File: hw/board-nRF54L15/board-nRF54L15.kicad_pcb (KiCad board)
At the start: 2 copper layers, 30 x 42 mm, 17 parts, among them J1 JST-PH 2.0 / BATTERY, SW1 B3U-1000P, U1 XIAO nRF54L15, U2 BMA400

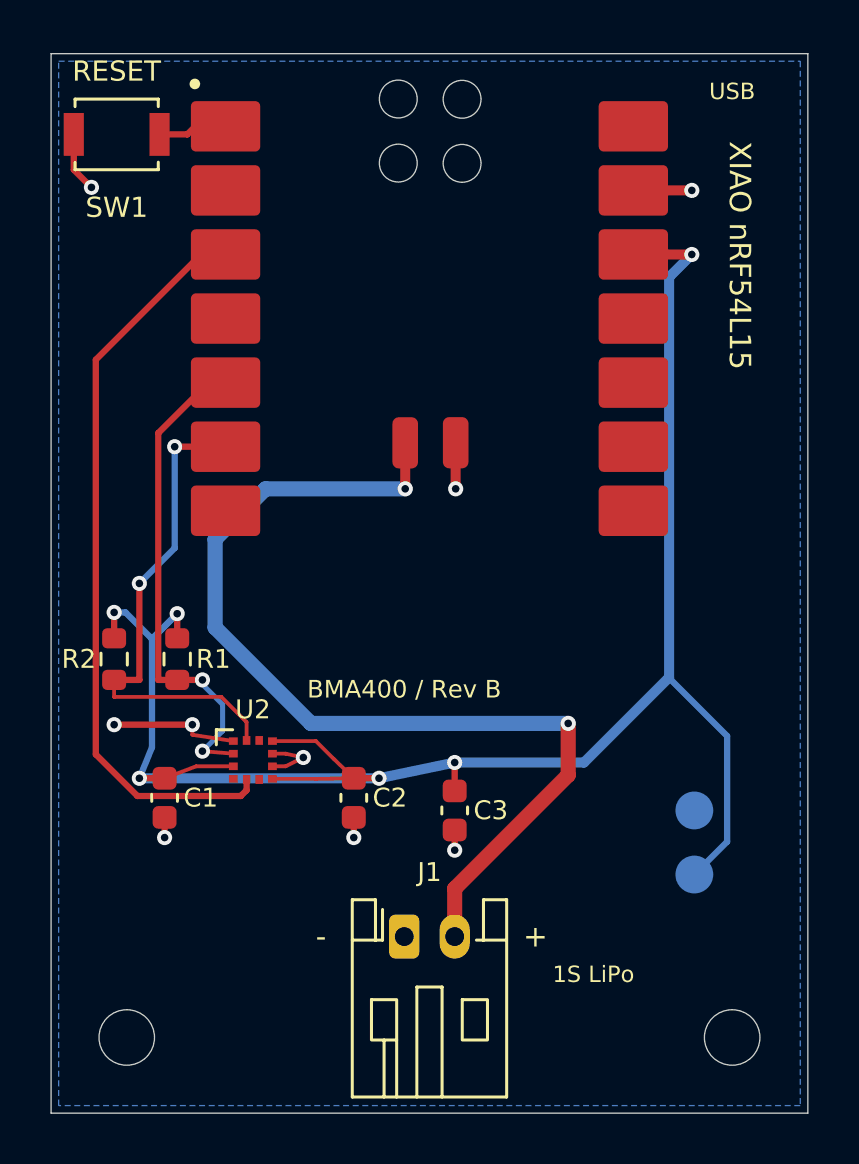
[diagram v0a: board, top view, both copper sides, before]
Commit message: Update PCB
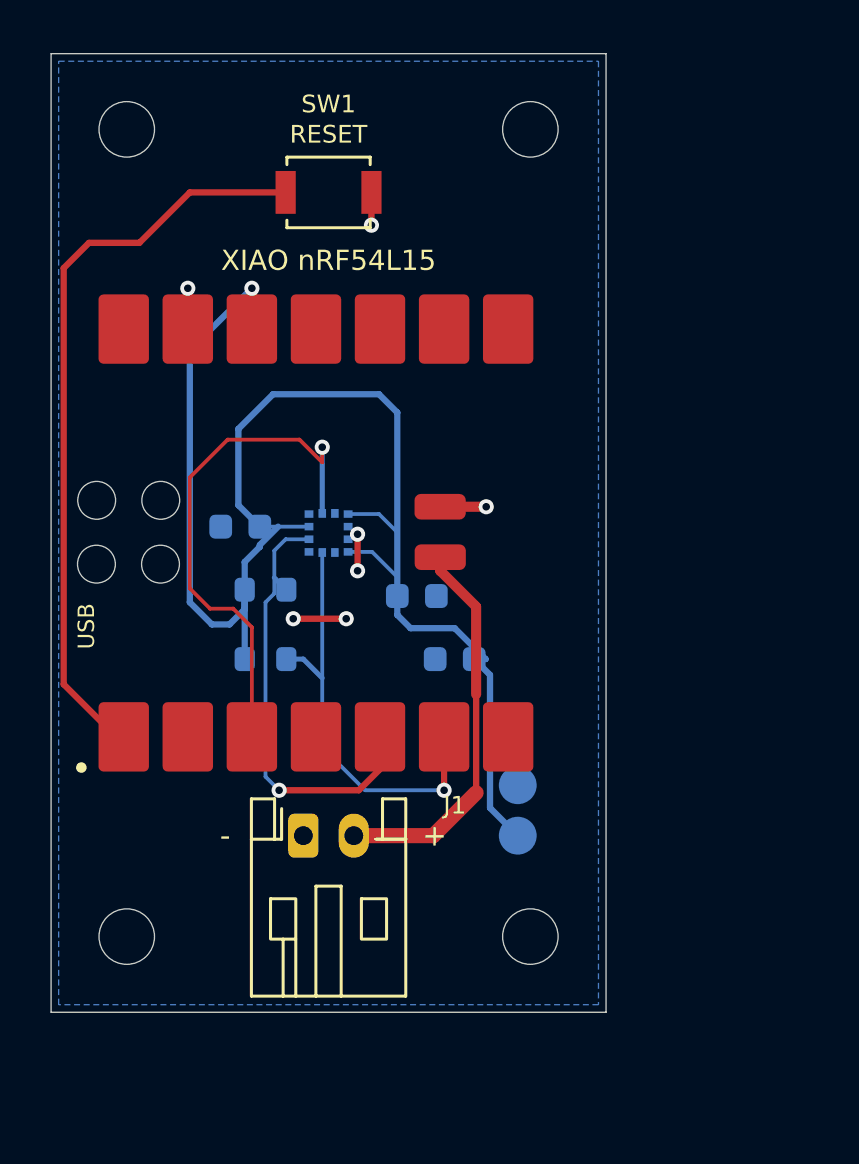
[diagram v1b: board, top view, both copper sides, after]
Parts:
- added H7: MountingHole_2.2mm_M2, Board:MountingHole_2.2mm_M2, F.Cu at (52.0, 53.0)
- added H8: MountingHole_2.2mm_M2, Board:MountingHole_2.2mm_M2, F.Cu at (68.0, 53.0)
- C1, C2, C3, R1, R2, U2: moved to B.Cu
- moved H3 22.0 mm to (50.8, 70.2), turned to 90 degrees
- moved H4 21.5 mm to (50.8, 67.7), turned to 90 degrees
- moved H5 18.5 mm to (53.3, 70.2), turned to 90 degrees
- moved H6 17.9 mm to (53.3, 67.7), turned to 90 degrees
- moved C1 11.2 mm to (56.5, 68.8), turned to 180 degrees
- moved U1 9.62 mm to (59.5, 69.0), turned to 90 degrees
- moved U2 9.49 mm to (60.0, 69.0)
- moved H2 8.94 mm to (68.0, 85.0)
- moved SW1 8.71 mm to (60.0, 55.5), turned to 0 degrees
- moved C2 8.38 mm to (63.5, 71.5), turned to 0 degrees
- moved TP1 7.17 mm to (67.5, 81.0)
- moved TP2 7.07 mm to (67.5, 79.0)
- moved C3 6.00 mm to (65.0, 74.0), turned to 180 degrees
- moved R2 6.00 mm to (57.5, 74.0), turned to 0 degrees
- moved J1 5.66 mm to (59.0, 81.0)
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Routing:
- net /FACTORY_RESET: track 2.75 -> 29.8 mm
- net /VBAT: track 39.6 -> 15.5 mm, vias 2 -> 0
- net /+3V3: track 76.6 -> 62.8 mm, vias 6 -> 1
- net /ACC_INT1: track 29.7 -> 21.3 mm, vias 0 -> 1
- net /GND: track 16.6 -> 8.29 mm, vias 9 -> 7
- net /I2C_SCL: track 19.9 -> 17.1 mm, vias 2 -> 1
- net /I2C_SDA: track 19.7 -> 17.7 mm, vias 2 -> 1
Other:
- board size 30 x 42 mm -> 22 x 38 mm
- board text added: "22 x 38 mm / 2 layers / 1.6 mm FR4"
- board text added: "BMA400 / Rev C"
- board text removed: "30 x 42 mm / 2 layers / 1.6 mm FR4"
- board text removed: "BMA400 / Rev B"
